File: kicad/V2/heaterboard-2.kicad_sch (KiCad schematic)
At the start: 12 parts, among them J1 Screw_Terminal_01x02, J2 Conn_01x05_Pin, J3 Conn_01x04_Pin, Q1 Q_NMOS_GDS, U1 LM317_TO-220

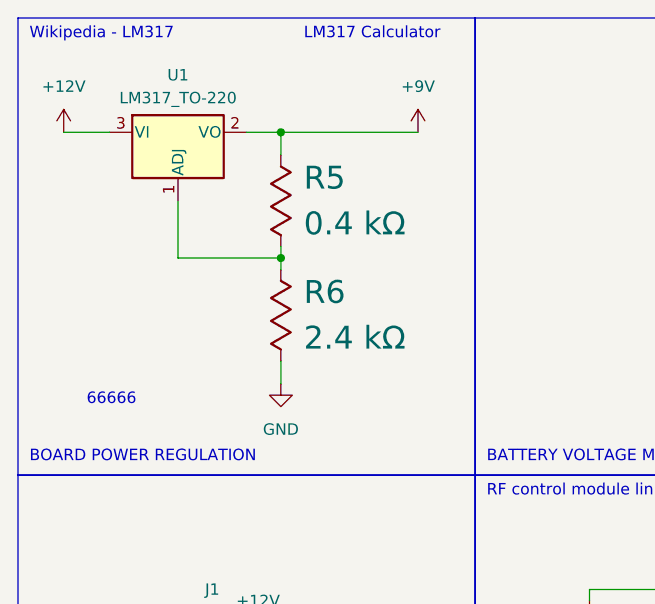
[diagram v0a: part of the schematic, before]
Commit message: end class02-06-2024
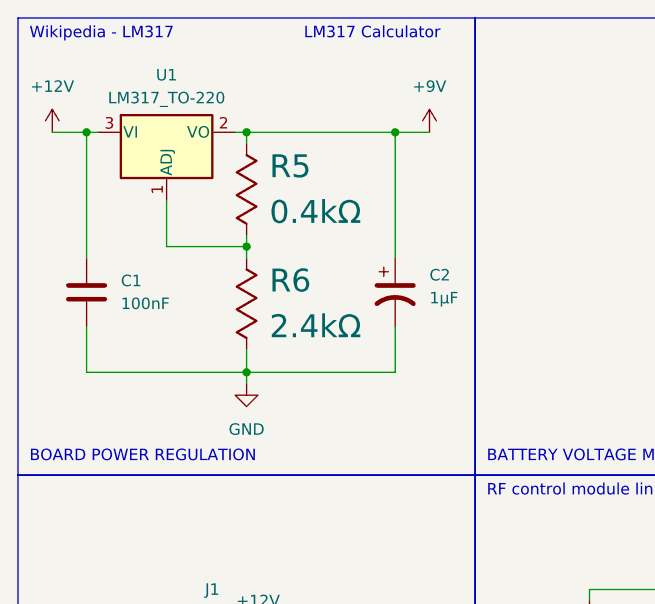
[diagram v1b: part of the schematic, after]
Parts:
- added C1: 100nF, symbol Device:C
- added C2: 1μF, symbol Device:C_Polarized_US
- R5: value 0.4 kΩ -> 0.4kΩ
- R6: value 2.4 kΩ -> 2.4kΩ
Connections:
- net +12V: now also C1.1
- net +9V: now also C2.1
- net GND: now also C1.2, C2.2
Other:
- note removed: "66666"
- moved on the sheet: R5, R6, U1

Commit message: pcb layout
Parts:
- C1, C2: footprint (none) -> Capacitor_THT:CP_Radial_D10.0mm_P5.00mm
- J1: footprint Connector_PinHeader_2.54mm:PinHeader_1x02_P2.54mm_Vertical -> TerminalBlock:TerminalBlock_Wuerth_691311400102_P7.62mm
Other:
- title: Windshield Heater -> Windshield Heater Controller Schematic
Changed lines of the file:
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@@
   (paper "USLetter")
   (title_block
-    (title "Windshield Heater")
+    (title "Windshield Heater Controller Schematic")
     (rev "2")
     (company "ME692")
@@
       (effects (font (size 1.27 1.27)) (justify left))
     )
-    (property "Footprint" "" (at 67.31 55.88 0)
+    (property "Footprint" "Capacitor_THT:CP_Radial_D10.0mm_P5.00mm" (at 67.31 55.88 0)
       (effects (font (size 1.27 1.27)) hide)
     )
@@
       (effects (font (size 1.27 1.27)) (justify left))
     )
-    (property "Footprint" "" (at 33.9852 59.69 0)
+    (property "Footprint" "Capacitor_THT:CP_Radial_D10.0mm_P5.00mm" (at 33.9852 59.69 0)
       (effects (font (size 1.27 1.27)) hide)
     )
@@
       (effects (font (size 1.27 1.27)))
     )
-    (property "Footprint" "Connector_PinHeader_2.54mm:PinHeader_1x02_P2.54mm_Vertical" (at 46.99 97.79 0)
-      (effects (font (size 1.27 1.27)) hide)
-    )
+    (property "Footprint" "TerminalBlock:TerminalBlock_Wuerth_691311400102_P7.62mm" (at 46.99 97.79 0)
+      (effects (font (size 1.27 1.27)) hide)
+    )
